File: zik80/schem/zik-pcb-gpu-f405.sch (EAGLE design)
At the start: 14 parts

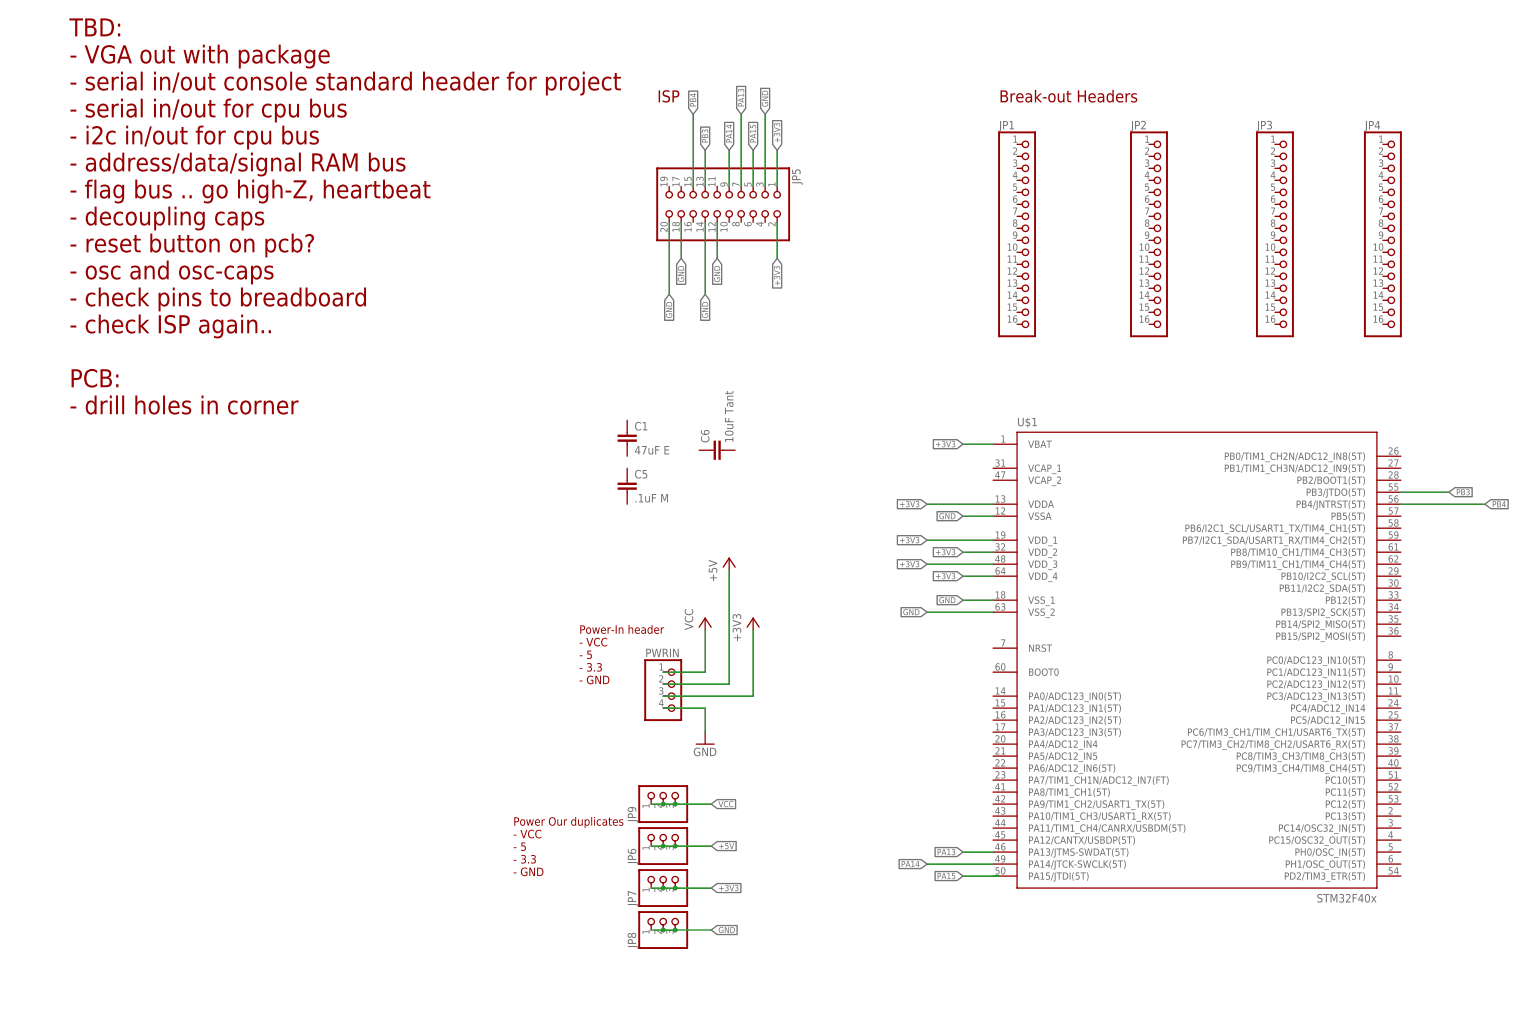
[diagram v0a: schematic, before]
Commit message: minor tweaks to gpu sche.. getting mentally ready for finishing it up, deciding what is pinheader versus actual footprints..
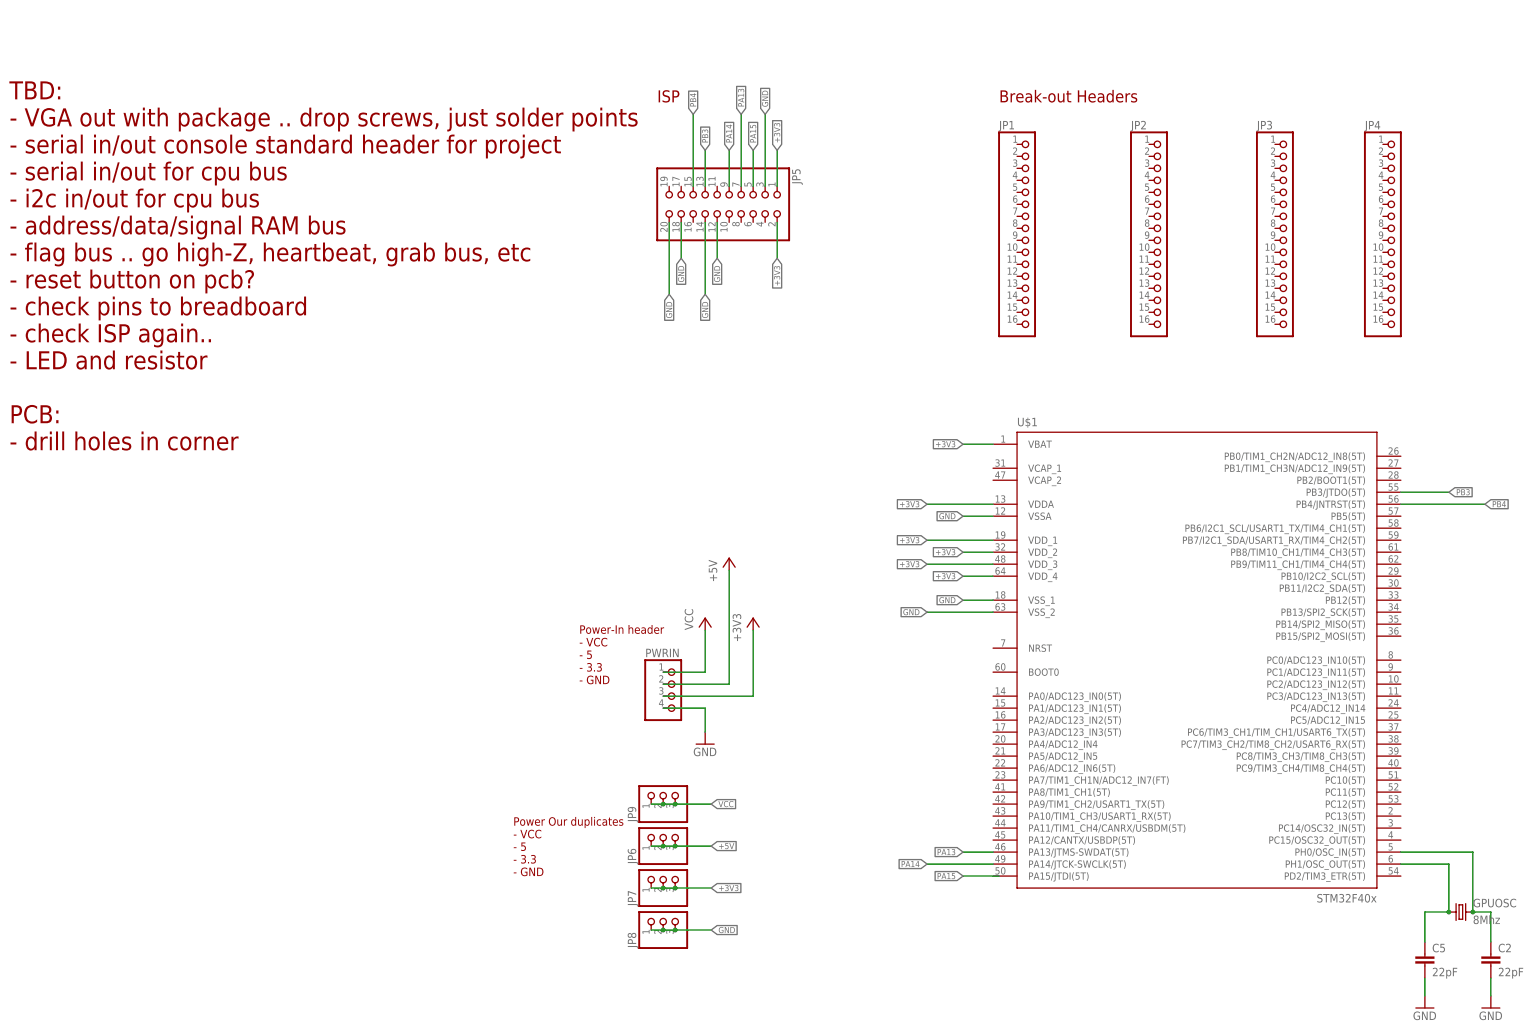
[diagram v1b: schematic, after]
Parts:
- removed C1: 47uF E, rcl:C-EU025-025X050
- removed C6: 10uF Tant, rcl:C-EU025-025X050
- added C2: 22pF, rcl:C-EU025-025X050
- added GPUOSC: 8Mhz, SparkFun-FreqCtrl:CRYSTALHC49US
- C5: value .1uF M -> 22pF
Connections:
- new net N$1: C5.1, GPUOSC.1, U$1.PH1/OSC_OUT(5T)
- new net N$2: C2.1, GPUOSC.2, U$1.PH0/OSC_IN(5T)
- net GND: now also C2.2, C5.2
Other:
- note added: "TBD: - VGA out with package .. drop screws, just solder points - serial in/out console standard header for project - serial in/out for cpu bus - i2c in/out for cpu bus - address/data/signal RAM bus - flag bus .. go high-Z, heartbeat, grab bus, etc - reset button on pcb? - check pins to breadboard - check ISP again.. - LED and resistor PCB: - drill holes in corner"
- note removed: "TBD: - VGA out with package - serial in/out console standard header for project - serial in/out for cpu bus - i2c in/out for cpu bus - address/data/signal RAM bus - flag bus .. go high-Z, heartbeat - decoupling caps - reset button on pcb? - osc and osc-caps - check pins to breadboard - check ISP again.. PCB: - drill holes in corner"
- moved on the sheet: C5
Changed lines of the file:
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@@
 <layer number="101" name="Patch_Top" color="12" fill="4" visible="yes" active="yes"/>
 <layer number="102" name="Vscore" color="7" fill="1" visible="yes" active="yes"/>
+<layer number="103" name="tMap" color="7" fill="1" visible="no" active="yes"/>
 <layer number="104" name="Name" color="7" fill="1" visible="yes" active="yes"/>
+<layer number="105" name="tPlate" color="7" fill="1" visible="no" active="yes"/>
+<layer number="106" name="bPlate" color="7" fill="1" visible="no" active="yes"/>
+<layer number="107" name="Crop" color="7" fill="1" visible="no" active="yes"/>
+<layer number="108" name="tplace-old" color="10" fill="1" visible="yes" active="yes"/>
+<layer number="109" name="ref-old" color="11" fill="1" visible="yes" active="yes"/>
 <layer number="116" name="Patch_BOT" color="9" fill="4" visible="yes" active="yes"/>
 <layer number="121" name="_tsilk" color="7" fill="1" visible="yes" active="yes"/>
 <layer number="122" name="_bsilk" color="7" fill="1" visible="yes" active="yes"/>
+<layer number="125" name="_tNames" color="7" fill="1" visible="no" active="yes"/>
+<layer number="144" name="Drill_legend" color="7" fill="1" visible="no" active="yes"/>
 <layer number="151" name="HeatSink" color="7" fill="1" visible="yes" active="yes"/>
+<layer number="199" name="Contour" color="7" fill="1" visible="yes" active="yes"/>
 <layer number="200" name="200bmp" color="1" fill="10" visible="no" active="no"/>
 <layer number="201" name="201bmp" color="2" fill="1" visible="no" active="no"/>
 <layer number="202" name="202bmp" color="3" fill="1" visible="no" active="no"/>
+<layer number="203" name="203bmp" color="4" fill="10" visible="no" active="yes"/>
+<layer number="204" name="204bmp" color="5" fill="10" visible="no" active="yes"/>
+<layer number="205" name="205bmp" color="6" fill="10" visible="no" active="yes"/>
+<layer number="206" name="206bmp" color="7" fill="10" visible="no" active="yes"/>
+<layer number="207" name="207bmp" color="8" fill="10" visible="no" active="yes"/>
+<layer number="208" name="208bmp" color="9" fill="10" visible="no" active="yes"/>
+<layer number="209" name="209bmp" color="7" fill="1" visible="no" active="yes"/>
+<layer number="210" name="210bmp" color="7" fill="1" visible="no" active="yes"/>
+<layer number="211" name="211bmp" color="7" fill="1" visible="no" active="yes"/>
+<layer number="212" name="212bmp" color="7" fill="1" visible="no" active="yes"/>
+<layer number="213" name="213bmp" color="7" fill="1" visible="no" active="yes"/>
+<layer number="214" name="214bmp" color="7" fill="1" visible="no" active="yes"/>
+<layer number="215" name="215bmp" color="7" fill="1" visible="no" active="yes"/>
+<layer number="216" name="216bmp" color="7" fill="1" visible="no" active="yes"/>
+<layer number="217" name="217bmp" color="18" fill="1" visible="no" active="no"/>
+<layer number="218" name="218bmp" color="19" fill="1" visible="no" active="no"/>
+<layer number="219" name="219bmp" color="20" fill="1" visible="no" active="no"/>
+<layer number="220" name="220bmp" color="21" fill="1" visible="no" active="no"/>
+<layer number="221" name="221bmp" color="22" fill="1" visible="no" active="no"/>
+<layer number="222" name="222bmp" color="23" fill="1" visible="no" active="no"/>
+<layer number="223" name="223bmp" color="24" fill="1" visible="no" active="no"/>
+<layer number="224" name="224bmp" color="25" fill="1" visible="no" active="no"/>
 <layer number="250" name="Descript" color="3" fill="1" visible="no" active="no"/>
 <layer number="251" name="SMDround" color="12" fill="11" visible="no" active="no"/>
@@
 <part name="+3V2" library="supply1" deviceset="+3V3" device=""/>
 <part name="PWRIN" library="pinhead" deviceset="PINHD-1X4" device=""/>
-<part name="C1" library="rcl" deviceset="C-EU" device="025-025X050" value="47uF E"/>
-<part name="C5" library="rcl" deviceset="C-EU" device="025-025X050" value=".1uF M"/>
-<part name="C6" library="rcl" deviceset="C-EU" device="025-025X050" value="10uF Tant"/>
+<part name="C5" library="rcl" deviceset="C-EU" device="025-025X050" value="22pF"/>
 <part name="U$1" library="stm32f4" deviceset="STM32F405R" device=""/>
 <part name="JP1" library="pinhead" deviceset="PINHD-1X16" device=""/>
@@
 <part name="JP8" library="pinhead" deviceset="PINHD-1X3" device=""/>
 <part name="JP9" library="pinhead" deviceset="PINHD-1X3" device=""/>
+<part name="GPUOSC" library="SparkFun-FreqCtrl" deviceset="CRYSTAL" device="HC49US" value="8Mhz"/>
+<part name="GND1" library="supply1" deviceset="GND" device=""/>
+<part name="GND2" library="supply1" deviceset="GND" device=""/>
+<part name="C2" library="rcl" deviceset="C-EU" device="025-025X050" value="22pF"/>
 </parts>
 <sheets>
@@
 - 3.3
 - GND</text>
-<text x="-121.92" y="64.77" size="3.81" layer="94">TBD:
-- VGA out with package
+<text x="-134.62" y="57.15" size="3.81" layer="94">TBD:
+- VGA out with package .. drop screws, just solder points
 - serial in/out console standard header for project
 - serial in/out for cpu bus
 - i2c in/out for cpu bus
 - address/data/signal RAM bus
-- flag bus .. go high-Z, heartbeat
-- decoupling caps
+- flag bus .. go high-Z, heartbeat, grab bus, etc
 - reset button on pcb?
-- osc and osc-caps
 - check pins to breadboard
 - check ISP again..
+- LED and resistor
 PCB:
 - drill holes in corner</text>
@@
 <instance part="+3V2" gate="G$1" x="22.86" y="21.59"/>
 <instance part="PWRIN" gate="A" x="6.35" y="5.08"/>
-<instance part="C1" gate="G$1" x="-3.81" y="60.96"/>
-<instance part="C5" gate="G$1" x="-3.81" y="50.8"/>
-<instance part="C6" gate="G$1" x="13.97" y="57.15" rot="R90"/>
+<instance part="C5" gate="G$1" x="165.1" y="-49.53"/>
 <instance part="U$1" gate="G$1" x="116.84" y="12.7"/>
 <instance part="JP1" gate="A" x="81.28" y="104.14"/>
@@
 <instance part="JP8" gate="A" x="3.81" y="-41.91" rot="R90"/>
 <instance part="JP9" gate="A" x="3.81" y="-15.24" rot="R90"/>
+<instance part="GPUOSC" gate="G$1" x="172.72" y="-40.64"/>
+<instance part="GND1" gate="1" x="165.1" y="-60.96"/>
+<instance part="GND2" gate="1" x="179.07" y="-60.96"/>
+<instance part="C2" gate="G$1" x="179.07" y="-49.53"/>
 </instances>
 <busses>
@@
 <label x="5.08" y="90.17" size="1.27" layer="95" rot="R270" xref="yes"/>
 </segment>
+<segment>
+<pinref part="C5" gate="G$1" pin="2"/>
+<pinref part="GND1" gate="1" pin="GND"/>
+<wire x1="165.1" y1="-58.42" x2="165.1" y2="-54.61" width="0.1524" layer="91"/>
+</segment>
+<segment>
+<pinref part="GND2" gate="1" pin="GND"/>
+<pinref part="C2" gate="G$1" pin="2"/>
+<wire x1="179.07" y1="-58.42" x2="179.07" y2="-54.61" width="0.1524" layer="91"/>
+</segment>
 </net>
 <net name="PA15" class="0">
@@
 </segment>
 </net>
+<net name="N$1" class="0">
+<segment>
+<pinref part="U$1" gate="G$1" pin="PH1/OSC_OUT(5T)"/>
+<pinref part="GPUOSC" gate="G$1" pin="1"/>
+<wire x1="160.02" y1="-30.48" x2="170.18" y2="-30.48" width="0.1524" layer="91"/>
+<wire x1="170.18" y1="-30.48" x2="170.18" y2="-40.64" width="0.1524" layer="91"/>
+<pinref part="C5" gate="G$1" pin="1"/>
+<wire x1="170.18" y1="-40.64" x2="165.1" y2="-40.64" width="0.1524" layer="91"/>
+<wire x1="165.1" y1="-40.64" x2="165.1" y2="-46.99" width="0.1524" layer="91"/>
+<junction x="170.18" y="-40.64"/>
+</segment>
+</net>
+<net name="N$2" class="0">
+<segment>
+<pinref part="U$1" gate="G$1" pin="PH0/OSC_IN(5T)"/>
+<pinref part="GPUOSC" gate="G$1" pin="2"/>
+<wire x1="160.02" y1="-27.94" x2="175.26" y2="-27.94" width="0.1524" layer="91"/>
+<wire x1="175.26" y1="-27.94" x2="175.26" y2="-40.64" width="0.1524" layer="91"/>
+<pinref part="C2" gate="G$1" pin="1"/>
+<wire x1="179.07" y1="-46.99" x2="179.07" y2="-40.64" width="0.1524" layer="91"/>
+<wire x1="179.07" y1="-40.64" x2="175.26" y2="-40.64" width="0.1524" layer="91"/>
+<junction x="175.26" y="-40.64"/>
+</segment>
+</net>

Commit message: Basic gpu pcb schem is done! Need to verify, and route, and good to go?
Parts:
- added C1, C4, C6, C7: .1uF, rcl:C-EU025-025X050
- added C3: ,1uF, rcl:C-EU025-025X050
- added C8, C9: 2.2uF, rcl:C-EU025-025X050
- added IOHDR, VGAHDR: (no value), pinhead:PINHD-1X6
- added LED1: (no value), SparkFun-LED:LED5MM
- added R1, R2, R3, R4, R5, R6, R7: (no value), rcl:R-US_0207/10
- added S1: SWITCH-MOMENTARY-2PTH, SparkFun-Electromechanical:SWITCH-MOMENTARY-2PTH
- added VIDEOHDR: (no value), pinhead:PINHD-1X8
- renumbered JP5 to ISPJTAG
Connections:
- removed net N$2: C2.1, GPUOSC.2, U$1.PH0/OSC_IN(5T)
- new net BOOT0: JP4.12, U$1.BOOT0
- new net N$10: VIDEOHDR.6
- new net N$3: LED1.A, R1.2
- new net N$5: R4.2, R5.2, VGAHDR.5
- new net N$8: R6.2, R7.2, VGAHDR.6
- new net NRST: JP1.7, S1.2, U$1.NRST
- new net PA0: JP1.14, U$1.PA0/ADC123_IN0(5T)
- new net PA1: JP1.15, U$1.PA1/ADC123_IN1(5T)
- new net PA10: JP3.11, U$1.PA10/TIM1_CH3/USART1_RX(5T), VIDEOHDR.3
- new net PA11: JP3.12, U$1.PA11/TIM1_CH4/CANRX/USBDM(5T)
- new net PA12: JP3.13, U$1.PA12/CANTX/USBDP(5T), VIDEOHDR.5
- new net PA2: JP1.16, U$1.PA2/ADC123_IN2(5T)
- new net PA3: JP2.1, U$1.PA3/ADC123_IN3(5T)
- new net PA4: JP2.4, U$1.PA4/ADC12_IN4
- new net PA5: JP2.5, U$1.PA5/ADC12_IN5
- new net PA6: JP2.6, U$1.PA6/ADC12_IN6(5T)
- new net PA7: JP2.7, U$1.PA7/TIM1_CH1N/ADC12_IN7(FT)
- new net PA8: JP3.9, U$1.PA8/TIM1_CH1(5T), VIDEOHDR.1
- new net PA9: JP3.10, U$1.PA9/TIM1_CH2/USART1_TX(5T), VIDEOHDR.2
- new net PB0: JP2.10, U$1.PB0/TIM1_CH2N/ADC12_IN8(5T)
- new net PB1: JP2.11, U$1.PB1/TIM1_CH3N/ADC12_IN9(5T)
- new net PB10: JP2.13, U$1.PB10/I2C2_SCL(5T), VGAHDR.1
- new net PB11: JP2.14, U$1.PB11/I2C2_SDA(5T), VGAHDR.2
- new net PB12: IOHDR.6, JP3.1, U$1.PB12(5T)
- new net PB13: JP3.2, U$1.PB13/SPI2_SCK(5T)
- new net PB14: JP3.3, U$1.PB14/SPI2_MISO(5T)
- new net PB15: JP3.4, U$1.PB15/SPI2_MOSI(5T)
- new net PB2: JP2.12, U$1.PB2/BOOT1(5T)
- new net PB5: JP4.9, U$1.PB5(5T)
- new net PB6: JP4.10, U$1.PB6/I2C1_SCL/USART1_TX/TIM4_CH1(5T), VIDEOHDR.7
- new net PB7: JP4.11, U$1.PB7/I2C1_SDA/USART1_RX/TIM4_CH2(5T), VIDEOHDR.8
- new net PB8: JP4.13, U$1.PB8/TIM10_CH1/TIM4_CH3(5T)
- new net PB9: JP4.14, U$1.PB9/TIM11_CH1/TIM4_CH4(5T)
- new net PC0: JP1.8, R3.1, U$1.PC0/ADC123_IN10(5T)
- new net PC1: JP1.9, R2.1, U$1.PC1/ADC123_IN11(5T)
- new net PC10: JP4.3, U$1.PC10(5T)
- new net PC11: JP4.4, U$1.PC11(5T)
- new net PC12: JP4.5, U$1.PC12(5T)
- new net PC13: JP1.2, U$1.PC13(5T)
- new net PC14: JP1.3, U$1.PC14/OSC32_IN(5T)
- new net PC15: JP1.4, U$1.PC15/OSC32_OUT(5T)
- new net PC2: JP1.10, R5.1, U$1.PC2/ADC123_IN12(5T)
- new net PC3: JP1.11, R4.1, U$1.PC3/ADC123_IN13(5T)
- new net PC4: JP2.8, R7.1, U$1.PC4/ADC12_IN14
- new net PC5: JP2.9, R6.1, U$1.PC5/ADC12_IN15
- new net PC6: IOHDR.1, JP3.5, U$1.PC6/TIM3_CH1/TIM_CH1/USART6_TX(5T)
- new net PC7: IOHDR.2, JP3.6, U$1.PC7/TIM3_CH2/TIM8_CH2/USART6_RX(5T)
- new net PC8: JP3.7, U$1.PC8/TIM3_CH3/TIM8_CH3(5T)
- new net PC9: JP3.8, U$1.PC9/TIM3_CH4/TIM8_CH4(5T)
- new net PD2: JP4.6, U$1.PD2/TIM3_ETR(5T)
- new net PH0: C2.1, GPUOSC.2, JP1.5, U$1.PH0/OSC_IN(5T)
- new net PH1: C5.1, GPUOSC.1, JP1.6, U$1.PH1/OSC_OUT(5T)
- new net VBAT: JP1.1, U$1.VBAT
- new net VCAP_1: C9.1, JP2.15, U$1.VCAP_1
- new net VCAP_2: C8.1, JP3.15, U$1.VCAP_2
- net +3V3: now also C1.1, C3.1, C4.1, C6.1, C7.1, JP1.13, JP2.16, JP2.3, JP3.16, JP4.16; no longer U$1.VBAT
- net +5V: now also R1.1
- net GND: now also C1.2, C3.2, C4.2, C6.2, C7.2, C8.2, C9.2, JP1.12, JP2.2, JP4.15, LED1.C, S1.1, VGAHDR.3
- net N$1: now also R2.2, R3.2; no longer C5.1, GPUOSC.1, U$1.PH1/OSC_OUT(5T)
- net PA13: now also JP3.14
- net PA14: now also JP4.1
- net PA15: now also JP4.2
- net PB3: now also JP4.7
- net PB4: now also JP4.8
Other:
- note added: "2.2uF = 22pF"
- note added: "Legend: + usart1 video + i2c p1: usart CK p2: TX p3: RX p4: CTS p5: RTS p6: p7: i2c scl p8: i2c sda"
- note added: "Legend: p1: Console TX (send from micro) p2: Console RX (receive to micro) p3: p4: p5: p6: vblank"
- note added: "Legend: p1: vsync: B10 p2: hsync: B11 p3: gnd p4: R p5: G p6: B"
- note added: "PC-low == RGB PB6/PB7 = i2c sda/scl ? conflict USART1? PB8 -> __? grab addr/data bus? PB9 -> __? heartbeat? PB10/11 == sync PB12 -> vblank __ = flags (hsync, vsync, heartbeat..) ?PC6-7 = console in/out .. use BoB jumpers PA8-PA12 = serial control in/out __ = address / data / control"
- note added: "Power LED 5V"
- note added: "Run to Vdd with .1uF decouple"
- note added: "TBD v2: - Add 2 brightness bits to VGA DAC - sync may need 80/100 resistor on some monitor - address/data/signal RAM bus"
- note added: "TBD: - check ISP again.. PCB: - drill holes in corner - version and website info - lavel +/-, and function points (hsync, vsync, etc)"
- note removed: "TBD: - VGA out with package .. drop screws, just solder points - serial in/out console standard header for project - serial in/out for cpu bus - i2c in/out for cpu bus - address/data/signal RAM bus - flag bus .. go high-Z, heartbeat, grab bus, etc - reset button on pcb? - check pins to breadboard - check ISP again.. - LED and resistor PCB: - drill holes in corner"
- moved on the sheet: PWRIN
